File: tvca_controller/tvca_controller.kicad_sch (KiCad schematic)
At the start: 21 parts, among them J1 Programming Header, J2 PT 1,5/ 4-5,0-H, U1 PIC18F26K83, U2 MCP2562, U3 INA180, Y1 Crystal 12 MHz

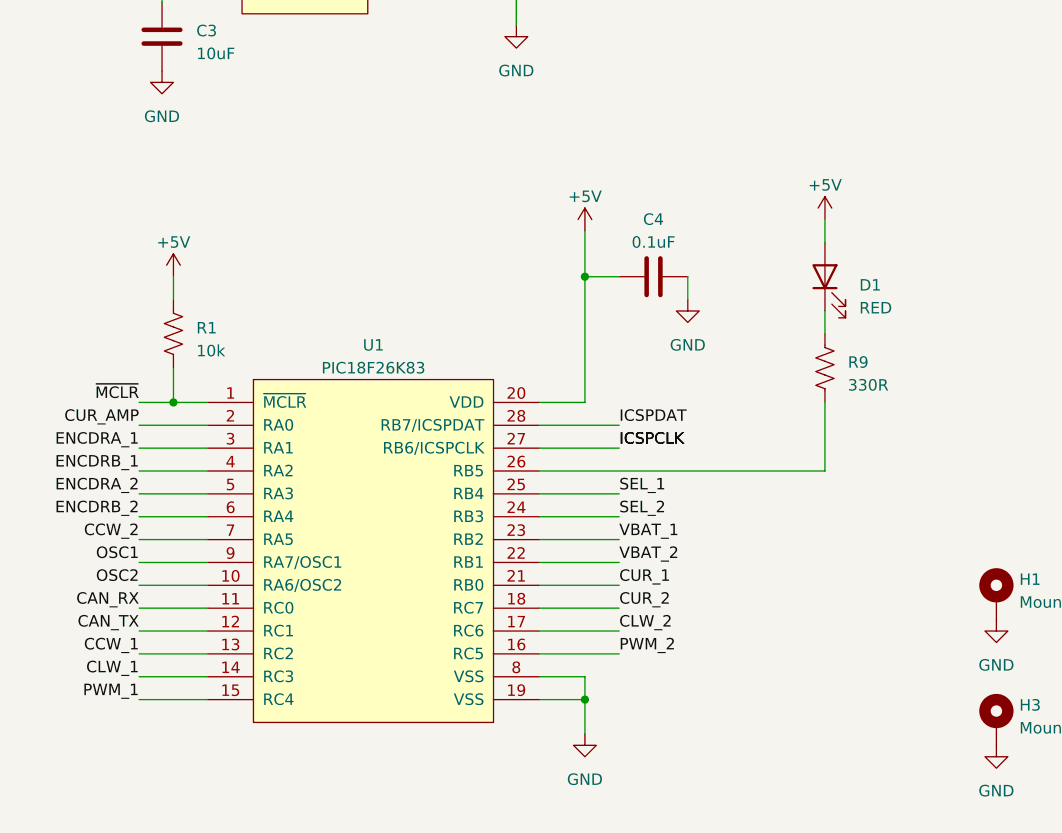
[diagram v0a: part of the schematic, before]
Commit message: routing
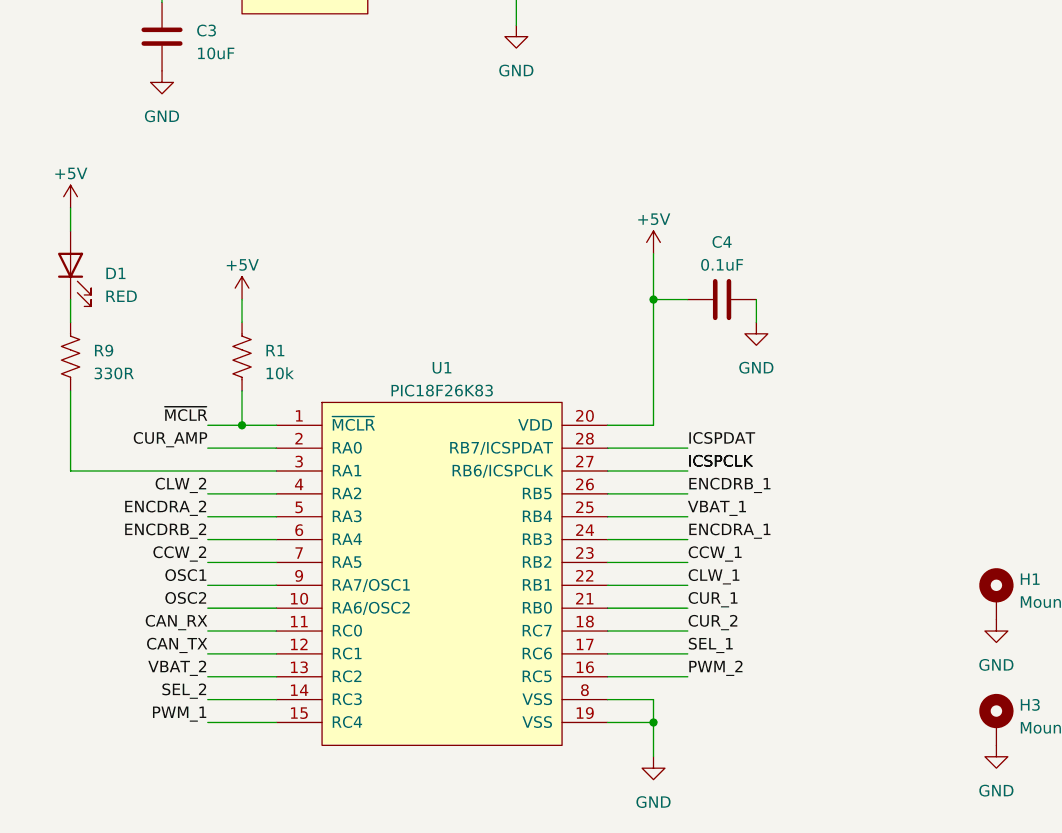
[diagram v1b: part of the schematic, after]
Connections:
- net CCW_1: now also U1.23 (RB2); no longer U1.13 (RC2)
- net CLW_1: now also U1.22 (RB1); no longer U1.14 (RC3)
- net CLW_2: now also U1.4 (RA2); no longer U1.17 (RC6)
- net ENCDRA_1: now also U1.24 (RB3); no longer U1.3 (RA1)
- net ENCDRB_1: now also U1.26 (RB5); no longer U1.4 (RA2)
- net SEL_1: now also U1.17 (RC6); no longer U1.25 (RB4)
- net SEL_2: now also U1.14 (RC3); no longer U1.24 (RB3)
- net VBAT_1: now also U1.25 (RB4); no longer U1.23 (RB2)
- net VBAT_2: now also U1.13 (RC2); no longer U1.22 (RB1)
- net at R9.1: now also U1.3 (RA1); no longer U1.26 (RB5)
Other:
- moved on the sheet: C4, D1, R1, R9, U1
